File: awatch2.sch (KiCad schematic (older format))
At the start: 0 parts

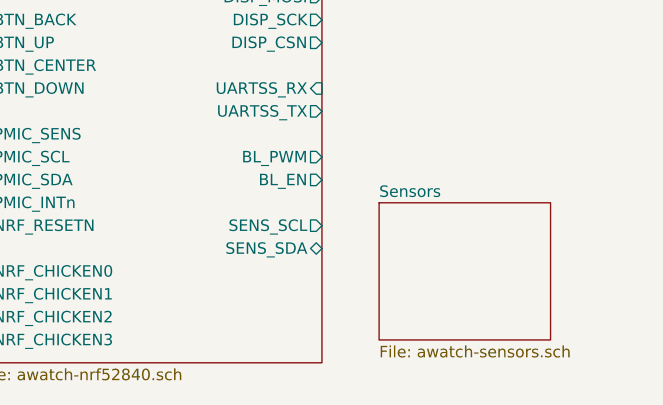
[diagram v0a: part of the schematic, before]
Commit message: add sensors
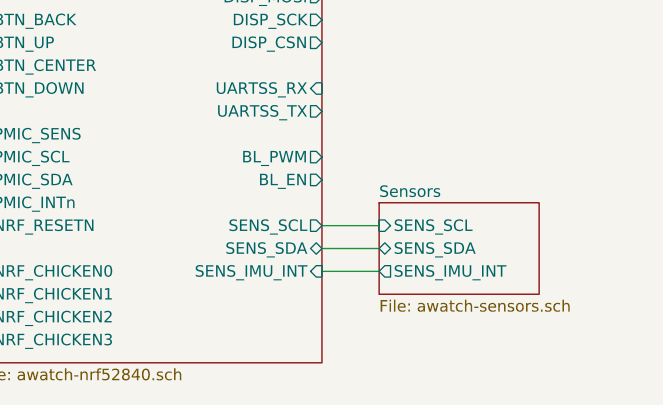
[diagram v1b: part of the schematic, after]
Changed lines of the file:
@@
 F35 "NRF_CHICKEN3" B L 3500 4400 50
 F36 "PMIC_INTn" I L 3500 3800 50
+F37 "SENS_IMU_INT" I R 5000 4100 50
 $EndSheet
 $Sheet
@@
 	5300 2300 5000 2300
 $Sheet
-S 5250 3800 750  600
+S 5250 3800 700  400
 U 5C3CD34E
 F0 "Sensors" 50
 F1 "awatch-sensors.sch" 50
+F2 "SENS_SCL" I L 5250 3900 50
+F3 "SENS_SDA" B L 5250 4000 50
+F4 "SENS_IMU_INT" O L 5250 4100 50
 $EndSheet
+Wire Wire Line
+	5250 3900 5000 3900
+Wire Wire Line
+	5250 4000 5000 4000
+Wire Wire Line
+	5250 4100 5000 4100
 $EndSCHEMATC
